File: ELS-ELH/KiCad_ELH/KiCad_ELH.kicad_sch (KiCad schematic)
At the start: 48 parts, among them Q1 IRLZ44N, Q3 IRLZ44N, Q4 IRLZ44N, Q5 IRLZ44N

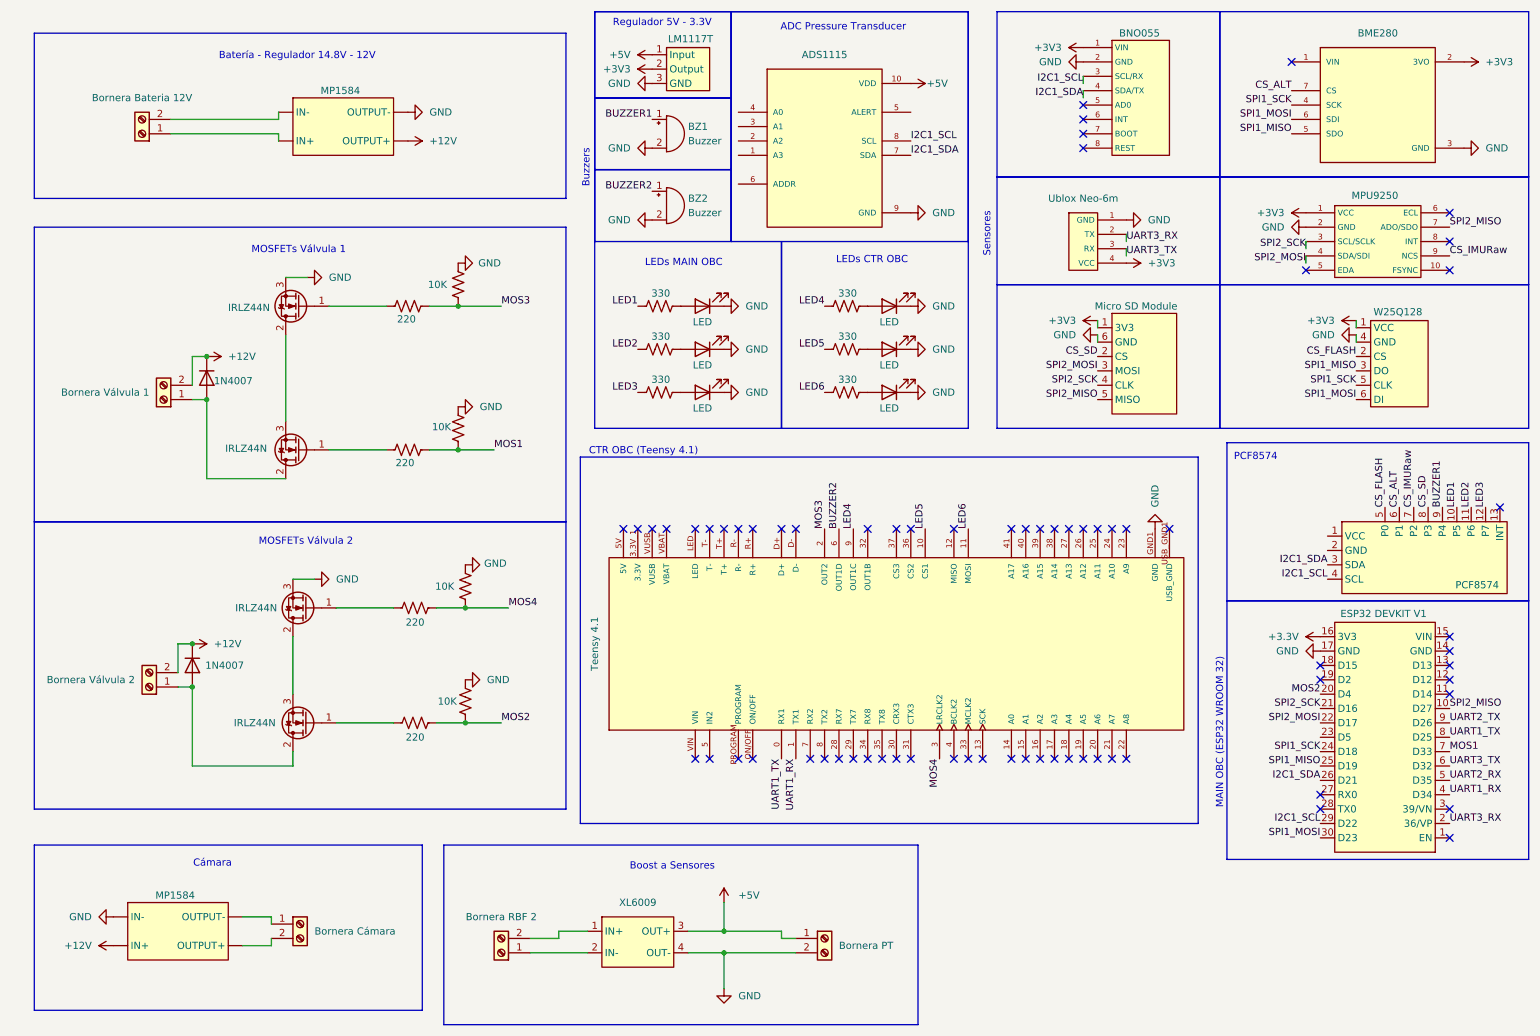
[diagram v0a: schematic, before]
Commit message: Finished schematics
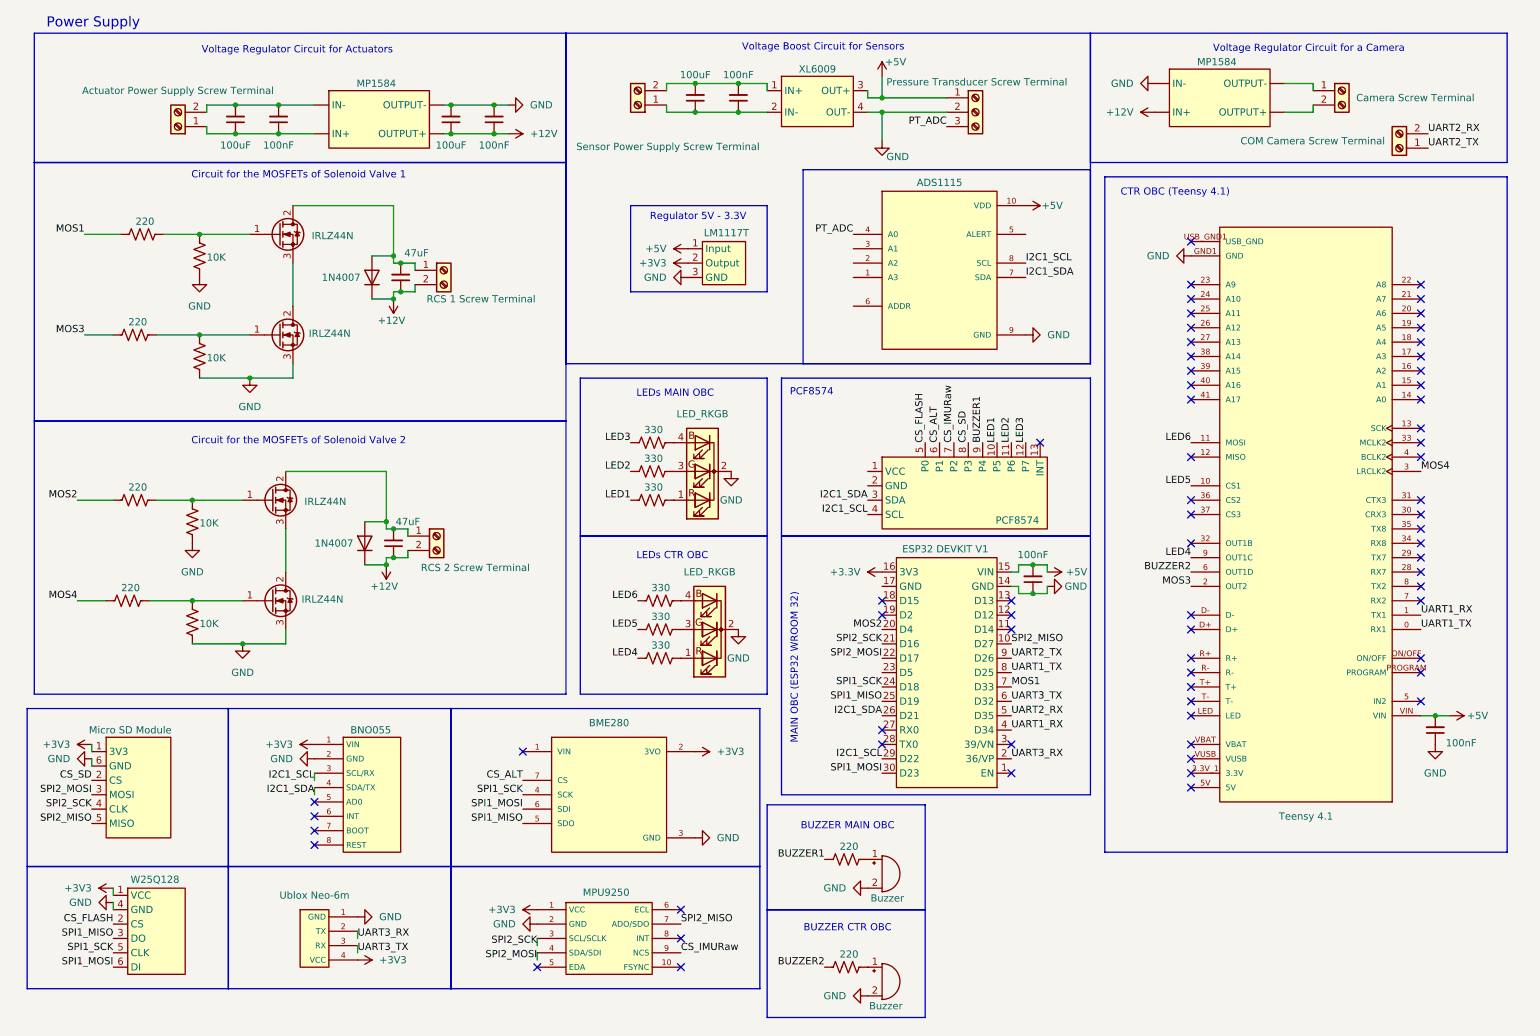
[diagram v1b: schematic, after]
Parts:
- removed Bornera2: Bornera PT, ELH_Library:Bornera 2P, symbol Connector:Screw_Terminal_01x02
- removed D2, D4, D5, D6, D7, D8: LED, ELH_Library:LED, symbol Device:LED
- removed D3: 1N4007, Diode_THT:D_DO-41_SOD81_P10.16mm_Horizontal, symbol Diode:1N4007
- removed Q3, Q5: IRLZ44N, Package_TO_SOT_THT:TO-220-3_Vertical, symbol Transistor_FET:IRLZ44N
- removed R13, R14: 330, Resistor_THT:R_Axial_DIN0207_L6.3mm_D2.5mm_P7.62mm_Horizontal, symbol Device:R_US
- added Bornera5: RCS 1 Screw Terminal, ELH_Library:Bornera 2P, symbol Connector:Screw_Terminal_01x02
- added C1, C2, C4, C6, C8: 100nF, symbol Device:C_Small
- added C10, C9: 47uF, symbol Device:C_Small
- added C3, C5, C7: 100uF, symbol Device:C_Small
- added D10, D3: LED_RKGB, LED_THT:LED_D5.0mm-4_RGB_Staggered_Pins, symbol Device:LED_RKGB
- added D9: 1N4007, Diode_THT:D_DO-41_SOD81_P10.16mm_Horizontal, symbol Diode:1N4007
- added J1: Pressure Transducer Screw Terminal, symbol Connector:Screw_Terminal_01x03
- added Q2, Q6: IRLZ44N, Package_TO_SOT_THT:TO-220-3_Vertical, symbol Transistor_FET:IRLZ44N
- added R16, R20: 220, Resistor_THT:R_Axial_DIN0207_L6.3mm_D2.5mm_P7.62mm_Horizontal, symbol Device:R_US
- added R18, R19: 10K, Resistor_THT:R_Axial_DIN0207_L6.3mm_D2.5mm_P7.62mm_Horizontal, symbol Device:R_US
- Bornera1: value Bornera RBF 2 -> Sensor Power Supply Screw Terminal
- Bornera3: value Bornera Cámara -> Camera Screw Terminal
- Bornera4: value Bornera Válvula 1 -> RCS 2 Screw Terminal
- Bornera6: value Bornera Bateria 12V -> Actuator Power Supply Screw Terminal
- Bornera7: value Bornera Válvula 2 -> COM Camera Screw Terminal
- R1: value 220 -> 330
- R11: value 220 -> 10K
- R12: value 330 -> 220
- R2, R8: value 10K -> 330
- R3: value 10K -> 220
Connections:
- net +12V: now also Bornera5.2 (Pin_2), C10.1, C7.1, C8.1, C9.1, D9.1 (K); no longer Bornera7.2 (Pin_2)
- net +5V: now also ESP1.15 (VIN), Teensy3.VIN, C1.2, C2.2, J1.1 (Pin_1)
- net BUZZER1: now also R12.1; no longer BZ1.1 (+)
- net BUZZER2: now also R9.1; no longer BZ2.1 (+)
- net GND: now also ESP1.14 (GND), R10.2, R11.2, C1.1, C2.1, C7.2, C8.2, D10.2 (K), D3.2 (K), J1.2 (Pin_2), Q2.3 (S), R18.2, R19.2; no longer ESP1.17 (GND), R10.1, R2.1, R3.2, R8.2
- net LED4: now also R8.2; no longer R12.2
- net LED5: now also R2.2
- net LED6: now also R1.2
- net MOS1: now also R16.1; no longer R3.1, R6.1
- net MOS2: now also R6.1; no longer R8.1, R9.1
- net MOS3: now also R20.1; no longer R10.2, R11.2
- net MOS4: now also R3.1; no longer R1.2, R2.2
- net UART2_RX: now also Bornera7.2 (Pin_2)
- net UART2_TX: now also Bornera7.1 (Pin_1)
- net at BOOST1.1 (IN+), Bornera1.2 (Pin_2): now also C5.2, C6.2
- net at BOOST1.2 (IN-), Bornera1.1 (Pin_1): now also C5.1, C6.1
- net at R4.1: now also D10.1 (RA)
- net at R5.1: now also D10.3 (GA)
- net at R1.1: now also D3.4 (BA)
- net at R7.1: now also D10.4 (BA)
- net at R9.2: now also BZ2.1 (+)
- net at Bornera6.1 (Pin_1), Regulator2. (OUTPUT+): now also C3.1, C4.1
- net at Bornera6.2 (Pin_2), Regulator2. (OUTPUT+): now also C3.2, C4.2
- net at Q4.1 (G), R11.1: now also R3.2
- net at Bornera4.1 (Pin_1), D1.2 (A), Q1.2 (D): now also C10.2
- net at Q1.1 (G), R6.2: now also R10.1
- net PT_ADC: now reaches ADC1.4 (A0)
- net PT_ADC: now also J1.3 (Pin_3)
- new net: Q6.1 (G), R16.2, R18.1
- new net: Bornera5.1 (Pin_1), C9.2, D9.2 (A), Q6.2 (D)
- new net: Q2.1 (G), R19.1, R20.2
- new net: D3.1 (RA), R8.1
- new net: D3.3 (GA), R2.1
- new net: Q2.2 (D), Q6.3 (S)
- new net: BZ1.1 (+), R12.2
- no-connect marks 70 -> 67
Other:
- note added: "BUZZER CTR OBC"
- note added: "BUZZER MAIN OBC"
- note added: "Circuit for the MOSFETs of Solenoid Valve 1"
- note added: "Circuit for the MOSFETs of Solenoid Valve 2"
- note added: "Power Supply"
- note added: "Regulator 5V - 3.3V"
- note added: "Voltage Boost Circuit for Sensors"
- note added: "Voltage Regulator Circuit for Actuators"
- note added: "Voltage Regulator Circuit for a Camera"
- note removed: "ADC Pressure Transducer"
- note removed: "Batería - Regulador 14.8V - 12V"
- note removed: "Boost a Sensores"
- note removed: "Buzzers"
- note removed: "Cámara"
- note removed: "MOSFETs Válvula 1"
- note removed: "MOSFETs Válvula 2"
- note removed: "Regulador 5V - 3.3V"
- note removed: "Sensores"
